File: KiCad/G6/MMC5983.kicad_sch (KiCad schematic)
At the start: 3 parts, among them U4 MMC5983MA-Magnetomer

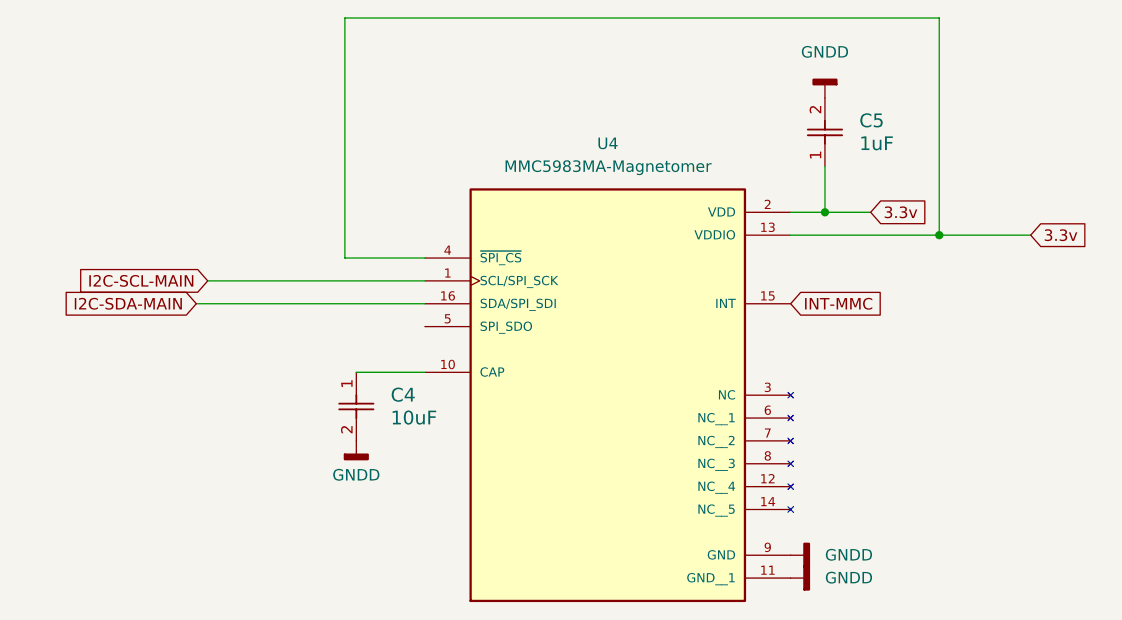
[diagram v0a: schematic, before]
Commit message: i finally finished routing everything to spi
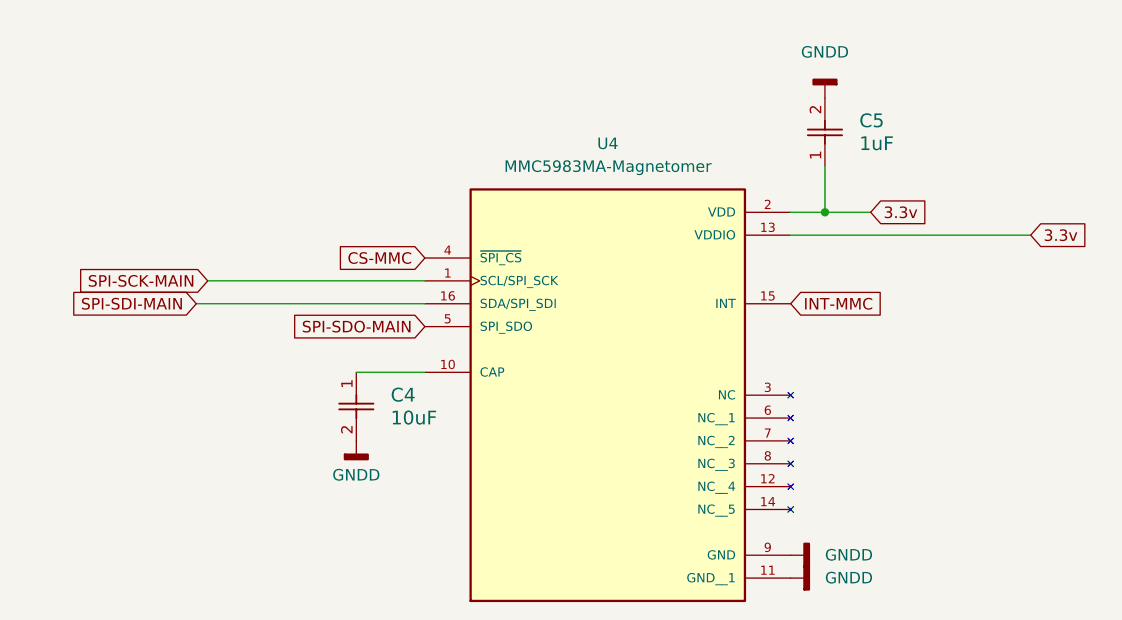
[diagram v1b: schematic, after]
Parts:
- C4: footprint CC0805KK7R7BB225:CAP_CC0805_YAG -> CC0603KRXQRQBB104:10CAPC370195_195N_KEM-L
- C5: footprint CC0603KRX7R7BB105:YAG_CC0603_YAG -> CC0603KRXQRQBB104:1CAP_CS1206_YAG
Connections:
- net 3.3v: no longer U4.4 (~{SPI_CS})
- net SPI-SDO-MAIN: now reaches U4.5 (SPI_SDO)
- net I2C-SCL-MAIN renamed SPI-SCK-MAIN
- net I2C-SDA-MAIN renamed SPI-SDI-MAIN
- new net CS-MMC: U4.4 (~{SPI_CS})
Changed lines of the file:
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@@
 	(paper "A4")
-	(junction
-		(at 171.45 83.82)
-		(diameter 0)
-		(color 0 0 0 0)
-	)
 	(junction
 		(at 158.75 81.28)
@@
 	(wire
 		(pts
-			(xy 154.94 83.82) (xy 171.45 83.82)
+			(xy 154.94 83.82) (xy 181.61 83.82)
 		)
 		(stroke
@@
 	(wire
 		(pts
-			(xy 105.41 59.69) (xy 105.41 86.36)
+			(xy 106.68 99.06) (xy 114.3 99.06)
 		)
 		(stroke
@@
 	(wire
 		(pts
-			(xy 106.68 99.06) (xy 114.3 99.06)
+			(xy 154.94 81.28) (xy 158.75 81.28)
 		)
 		(stroke
@@
 	(wire
 		(pts
-			(xy 154.94 81.28) (xy 158.75 81.28)
+			(xy 158.75 76.2) (xy 158.75 81.28)
 		)
 		(stroke
@@
 	(wire
 		(pts
-			(xy 171.45 59.69) (xy 171.45 83.82)
+			(xy 90.17 88.9) (xy 114.3 88.9)
 		)
 		(stroke
@@
 	(wire
 		(pts
-			(xy 171.45 83.82) (xy 181.61 83.82)
+			(xy 158.75 81.28) (xy 163.83 81.28)
 		)
 		(stroke
@@
 		)
 	)
-	(wire
-		(pts
-			(xy 158.75 76.2) (xy 158.75 81.28)
-		)
-		(stroke
-			(width 0)
-			(type default)
-		)
-	)
-	(wire
-		(pts
-			(xy 90.17 88.9) (xy 114.3 88.9)
-		)
-		(stroke
-			(width 0)
-			(type default)
-		)
-	)
-	(wire
-		(pts
-			(xy 105.41 86.36) (xy 114.3 86.36)
-		)
-		(stroke
-			(width 0)
-			(type default)
-		)
-	)
-	(wire
-		(pts
-			(xy 158.75 81.28) (xy 163.83 81.28)
-		)
-		(stroke
-			(width 0)
-			(type default)
-		)
-	)
-	(wire
-		(pts
-			(xy 105.41 59.69) (xy 171.45 59.69)
-		)
-		(stroke
-			(width 0)
-			(type default)
-		)
-	)
-	(global_label "I2C-SDA-MAIN"
+	(global_label "SPI-SDI-MAIN"
 		(shape input)
 		(at 88.9 91.44 180)
@@
 		)
 		(property "Intersheetrefs" "${INTERSHEET_REFS}"
-			(at 71.6423 91.44 0)
+			(at 72.1261 91.44 0)
 			(effects
 				(font
@@
 		)
 	)
-	(global_label "I2C-SCL-MAIN"
+	(global_label "SPI-SCK-MAIN"
 		(shape input)
 		(at 90.17 88.9 180)
@@
 		)
 		(property "Intersheetrefs" "${INTERSHEET_REFS}"
-			(at 72.9728 88.9 0)
+			(at 72.7309 88.9 0)
+			(effects
+				(font
+					(size 1.27 1.27)
+				)
+				(justify right)
+				(hide yes)
+			)
+		)
+	)
+	(global_label "SPI-SDO-MAIN"
+		(shape input)
+		(at 114.3 93.98 180)
+		(fields_autoplaced yes)
+		(effects
+			(font
+				(size 1.27 1.27)
+			)
+			(justify right)
+		)
+		(property "Intersheetrefs" "${INTERSHEET_REFS}"
+			(at 96.8004 93.98 0)
 			(effects
 				(font
@@
 				)
 				(justify left)
+				(hide yes)
+			)
+		)
+	)
+	(global_label "CS-MMC"
+		(shape input)
+		(at 114.3 86.36 180)
+		(fields_autoplaced yes)
+		(effects
+			(font
+				(size 1.27 1.27)
+			)
+			(justify right)
+		)
+		(property "Intersheetrefs" "${INTERSHEET_REFS}"
+			(at 103.0901 86.36 0)
+			(effects
+				(font
+					(size 1.27 1.27)
+				)
+				(justify right)
 				(hide yes)
 			)
@@
 			)
 		)
-		(property "Footprint" "CC0805KK7R7BB225:CAP_CC0805_YAG"
+		(property "Footprint" "CC0603KRXQRQBB104:10CAPC370195_195N_KEM-L"
 			(at 106.68 99.06 0)
 			(effects
@@
 			)
 		)
-		(property "Footprint" "CC0603KRX7R7BB105:YAG_CC0603_YAG"
+		(property "Footprint" "CC0603KRXQRQBB104:1CAP_CS1206_YAG"
 			(at 158.75 76.2 0)
 			(effects

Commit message: uhhhh im confused gang
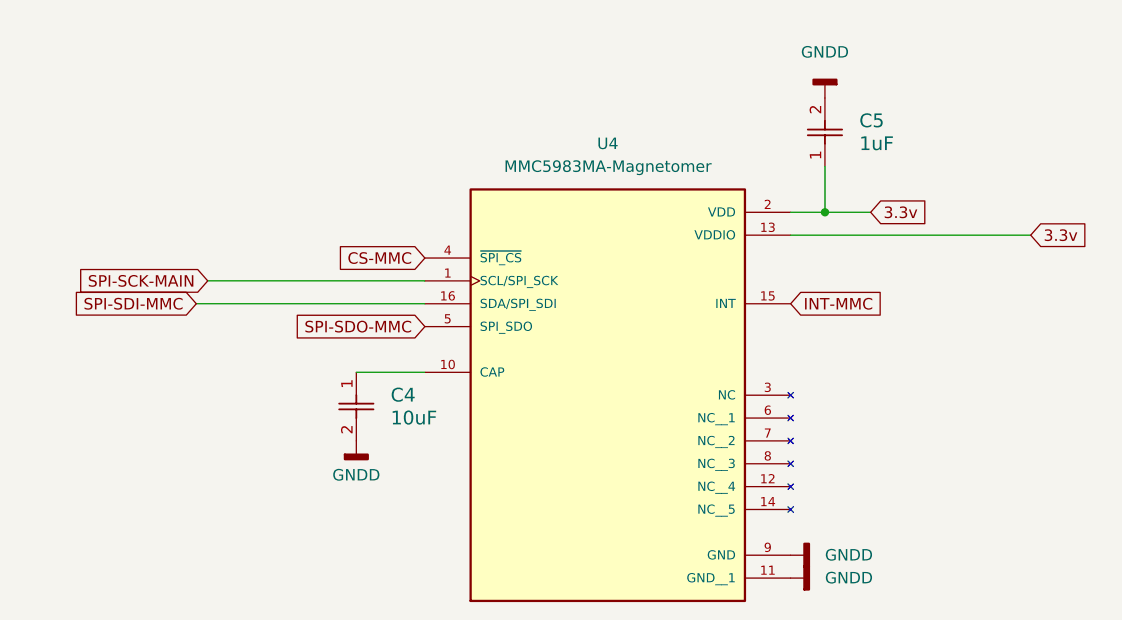
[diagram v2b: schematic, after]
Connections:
- net SPI-SDI-MAIN renamed SPI-SDI-MMC
- net SPI-SDO-MAIN renamed SPI-SDO-MMC
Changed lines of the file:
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@@
 		)
 	)
-	(global_label "SPI-SDI-MAIN"
+	(global_label "SPI-SDI-MMC"
 		(shape input)
 		(at 88.9 91.44 180)
@@
 		)
 		(property "Intersheetrefs" "${INTERSHEET_REFS}"
-			(at 72.1261 91.44 0)
+			(at 72.4286 91.44 0)
 			(effects
 				(font
@@
 		)
 	)
-	(global_label "SPI-SDO-MAIN"
+	(global_label "SPI-SDO-MMC"
 		(shape input)
 		(at 114.3 93.98 180)
@@
 		)
 		(property "Intersheetrefs" "${INTERSHEET_REFS}"
-			(at 96.8004 93.98 0)
+			(at 97.1029 93.98 0)
 			(effects
 				(font

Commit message: I think the schematics done uhhh idrk
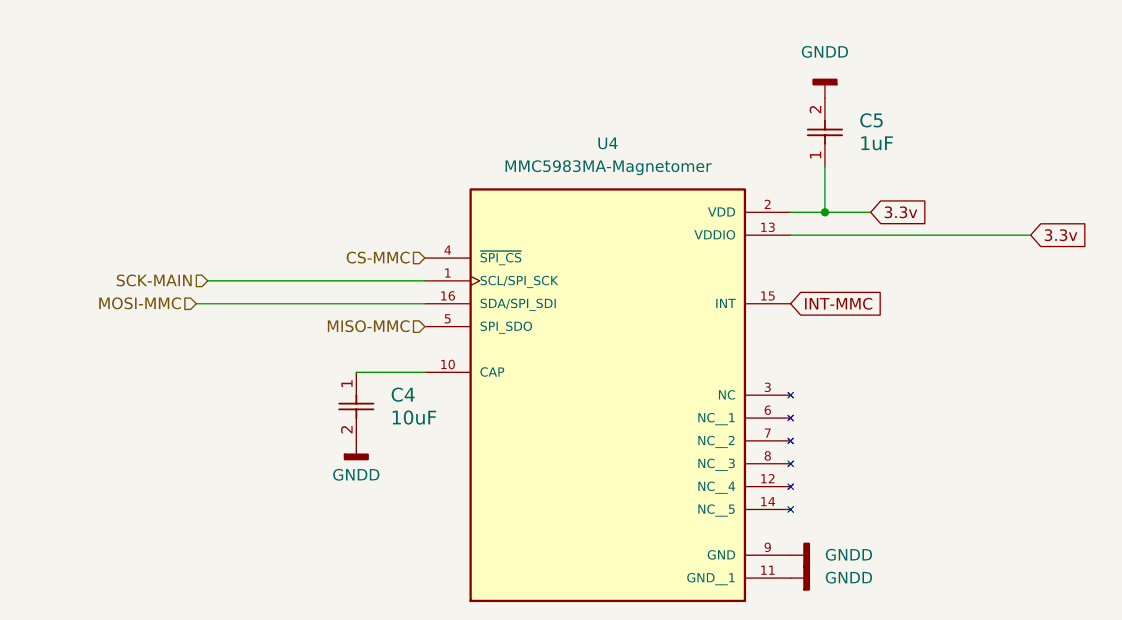
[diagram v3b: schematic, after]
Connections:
- net SPI-SCK-MAIN renamed SCK-MAIN
- net SPI-SDI-MMC renamed MOSI-MMC
- net SPI-SDO-MMC renamed MISO-MMC
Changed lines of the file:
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@@
-		)
-	)
-	(global_label "SPI-SDI-MMC"
-		(shape input)
-		(at 88.9 91.44 180)
-		(fields_autoplaced yes)
-		(effects
-			(font
-				(size 1.27 1.27)
-			)
-			(justify right)
-		)
-		(property "Intersheetrefs" "${INTERSHEET_REFS}"
-			(at 72.4286 91.44 0)
-			(effects
-				(font
-					(size 1.27 1.27)
-				)
-				(justify right)
-				(hide yes)
-			)
 		)
 	)
@@
 				)
 				(justify left)
-				(hide yes)
-			)
-		)
-	)
-	(global_label "SPI-SCK-MAIN"
-		(shape input)
-		(at 90.17 88.9 180)
-		(fields_autoplaced yes)
-		(effects
-			(font
-				(size 1.27 1.27)
-			)
-			(justify right)
-		)
-		(property "Intersheetrefs" "${INTERSHEET_REFS}"
-			(at 72.7309 88.9 0)
-			(effects
-				(font
-					(size 1.27 1.27)
-				)
-				(justify right)
-				(hide yes)
-			)
-		)
-	)
-	(global_label "SPI-SDO-MMC"
-		(shape input)
-		(at 114.3 93.98 180)
-		(fields_autoplaced yes)
-		(effects
-			(font
-				(size 1.27 1.27)
-			)
-			(justify right)
-		)
-		(property "Intersheetrefs" "${INTERSHEET_REFS}"
-			(at 97.1029 93.98 0)
-			(effects
-				(font
-					(size 1.27 1.27)
-				)
-				(justify right)
 				(hide yes)
 			)
@@
 		)
 	)
-	(global_label "CS-MMC"
+	(hierarchical_label "SCK-MAIN"
 		(shape input)
-		(at 114.3 86.36 180)
-		(fields_autoplaced yes)
+		(at 90.17 88.9 180)
 		(effects
 			(font
@@
 			(justify right)
 		)
-		(property "Intersheetrefs" "${INTERSHEET_REFS}"
-			(at 103.0901 86.36 0)
-			(effects
-				(font
-					(size 1.27 1.27)
-				)
-				(justify right)
-				(hide yes)
+	)
+	(hierarchical_label "MOSI-MMC"
+		(shape input)
+		(at 88.9 91.44 180)
+		(effects
+			(font
+				(size 1.27 1.27)
 			)
+			(justify right)
 		)
 	)
+	(hierarchical_label "MISO-MMC"
+		(shape input)
+		(at 114.3 93.98 180)
+		(effects
+			(font
+				(size 1.27 1.27)
+			)
+			(justify right)
+		)
+	)
+	(hierarchical_label "CS-MMC"
+		(shape input)
+		(at 114.3 86.36 180)
+		(effects
+			(font
+				(size 1.27 1.27)
+			)
+			(justify right)
+		)
+	)
